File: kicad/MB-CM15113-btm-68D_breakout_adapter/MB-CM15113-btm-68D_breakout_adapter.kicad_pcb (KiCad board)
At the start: 2 copper layers, 31.7 x 43.3 mm, 4 parts, among them P1 CONN_01X16, P2 CONN_01X05, P3 CONN_01X16, U1 MB-CM15113

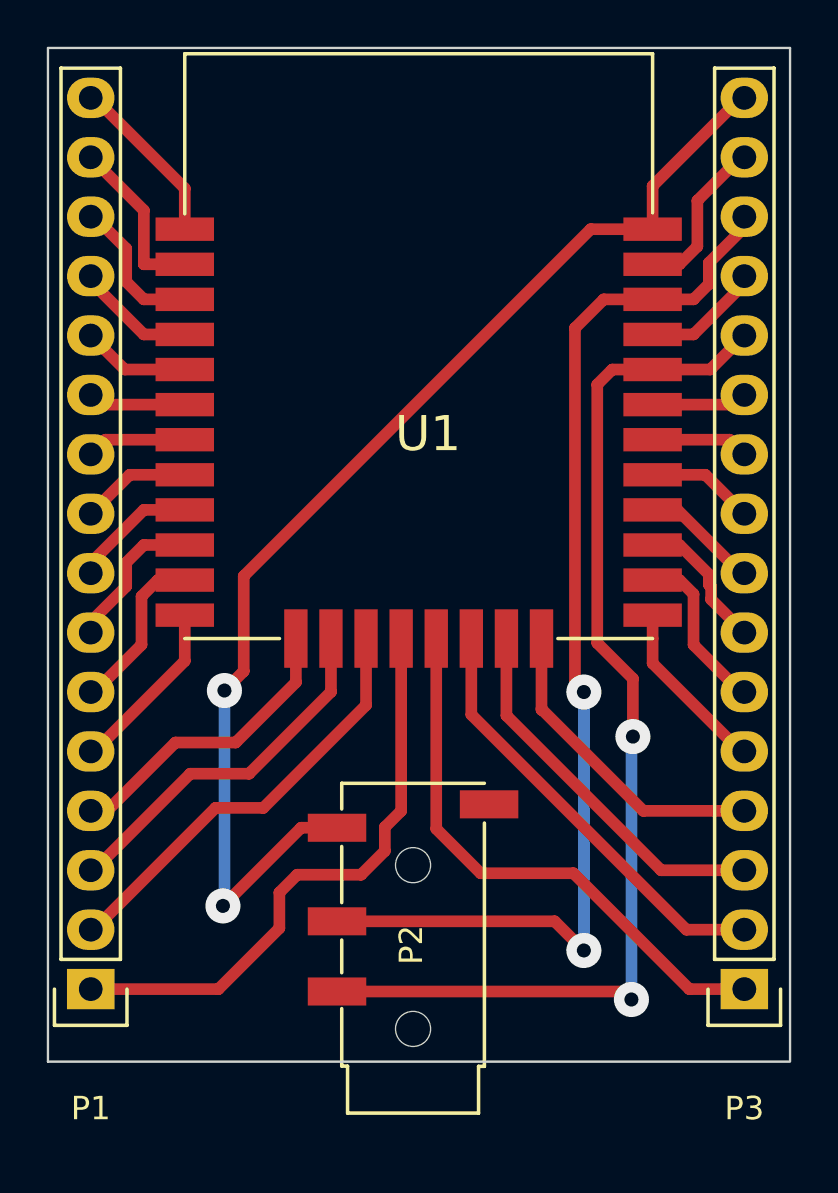
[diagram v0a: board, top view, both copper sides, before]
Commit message: udpates
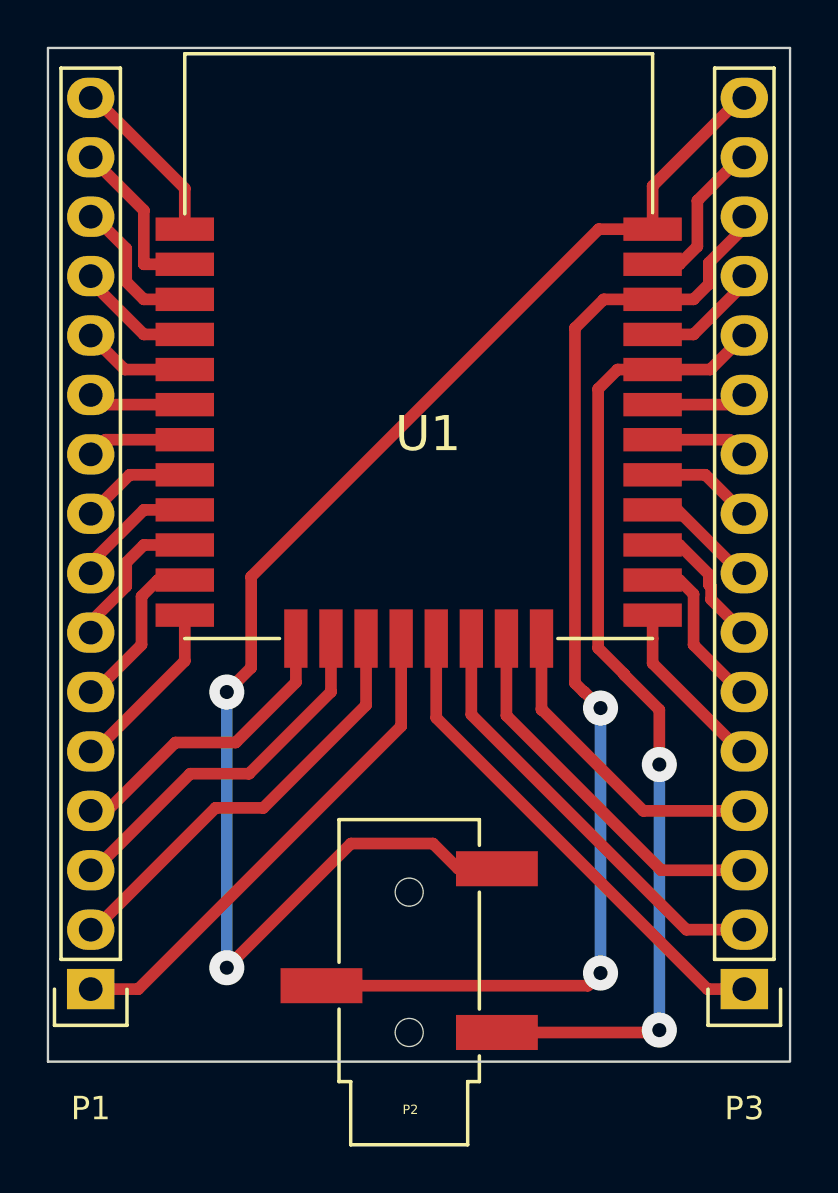
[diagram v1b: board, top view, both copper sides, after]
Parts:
- P2: footprint jacks:PJ3020D -> jacks:3.5mm_stereo_jack_PJ320B
- moved P2 1.46 mm to (158.4, 127.6)
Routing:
- net Net-(P2-Pad5): track 51.7 -> 62.0 mm
- net Net-(P2-Pad1): track 46.8 -> 42.7 mm
- net Net-(P3-Pad1): track 25.1 -> 21.4 mm
- net Net-(P1-Pad1): track 25.4 -> 21.8 mm
- net Net-(P2-Pad2): track 47.8 -> 50.2 mm
